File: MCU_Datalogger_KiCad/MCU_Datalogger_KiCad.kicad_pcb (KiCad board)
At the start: 2 copper layers, 50.8 x 30.5 mm, 29 parts, among them J1 Conn_01x04_Male, J2 Conn_01x04_Male, J3 Conn_01x09_Male, J4 Conn_02x03_Odd_Even, U1 24LC1025, U2 DS1337S+, U3 24LC1025, U4 ATMEGA328P-AU, Y1 32.768 KHz, Y2 16 MHz

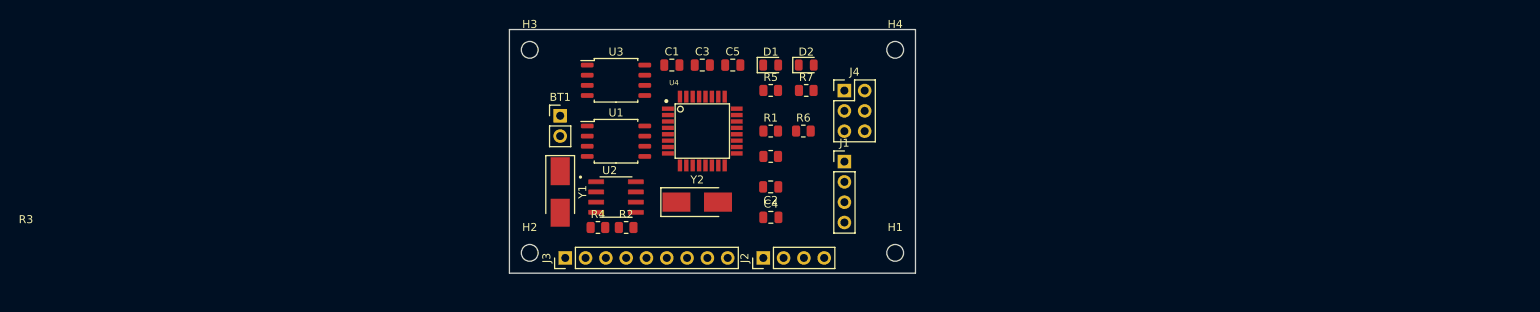
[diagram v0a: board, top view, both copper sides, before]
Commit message: Routing
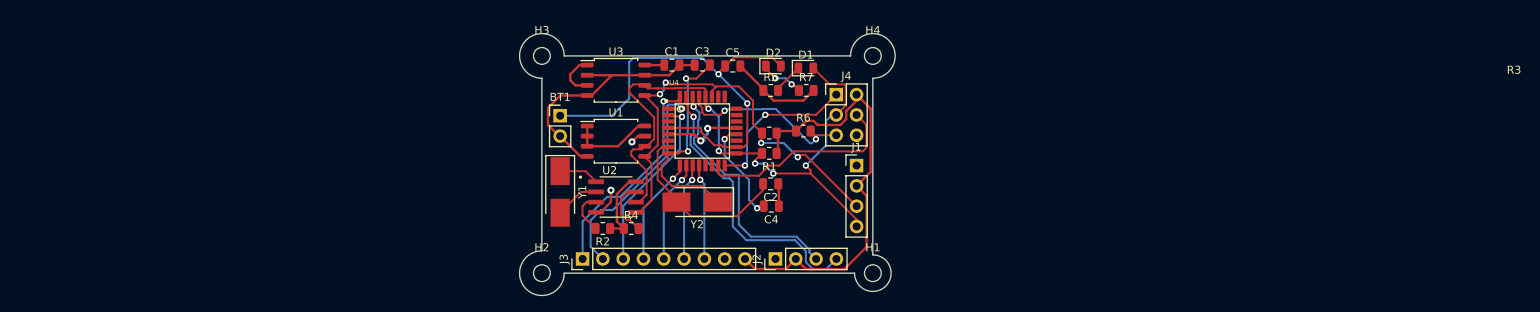
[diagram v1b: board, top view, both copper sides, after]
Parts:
- moved D1 4.41 mm to (62.5, 42.9)
- moved R4 4.17 mm to (40.6, 63.0)
- moved D2 4.11 mm to (58.4, 42.7)
- moved H1 3.78 mm to (70.9, 68.6)
- moved H2 2.96 mm to (29.5, 68.6)
- moved R3 2.93 mm to (57.9, 51.1), turned to 180 degrees
- moved R2 2.92 mm to (37.1, 63.0), turned to 180 degrees
- moved H4 2.90 mm to (70.9, 41.4)
- moved R1 2.80 mm to (57.9, 53.6), turned to 180 degrees
- moved J3 2.17 mm to (34.6, 66.8)
- moved H3 1.70 mm to (29.5, 41.4)
- moved J1 1.60 mm to (68.8, 55.1)
- moved J2 1.53 mm to (58.7, 66.8)
- moved C4 1.40 mm to (58.2, 60.2), turned to 180 degrees
- moved J4 1.14 mm to (66.3, 46.2)
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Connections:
- D1 pad 2: /SDK -> /SCK
- U4 pad 17: /SDK -> /SCK
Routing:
- net /Vcc: track 0.00 -> 84.1 mm
- net /SCK: track 0.00 -> 80.0 mm, vias 0 -> 5
- net GND: track 0.00 -> 63.7 mm, vias 0 -> 4
- net Net-(BT1-Pad1): track 0.00 -> 57.2 mm, vias 0 -> 2
- net /SDA: track 0.00 -> 55.9 mm, vias 0 -> 4
- net /TX: track 0.00 -> 35.2 mm, vias 0 -> 1
- net /RX: track 0.00 -> 32.1 mm, vias 0 -> 1
- net /D3: track 0.00 -> 28.5 mm, vias 0 -> 1
- net /D2: track 0.00 -> 27.4 mm, vias 0 -> 1
- net Net-(C3-Pad2): track 0.00 -> 27.1 mm, vias 0 -> 2
- net /MOSI: track 0.00 -> 26.4 mm
- net /RESET: track 0.00 -> 23.5 mm, vias 0 -> 2
- net Net-(C2-Pad2): track 0.00 -> 22.6 mm
- net /D4: track 0.00 -> 22.1 mm, vias 0 -> 1
- net /MISO: track 0.00 -> 19.9 mm, vias 0 -> 2
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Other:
- board size 50.8 x 30.5 mm -> 47 x 32.8 mm
